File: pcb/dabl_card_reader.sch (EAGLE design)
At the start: 11 parts

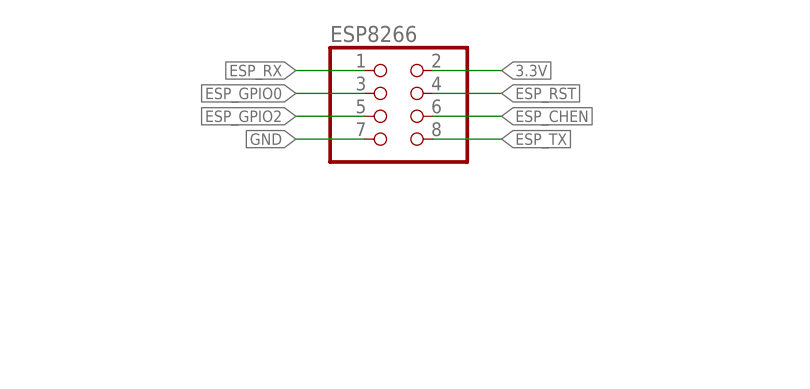
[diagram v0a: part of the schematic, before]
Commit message: fix pcb traces
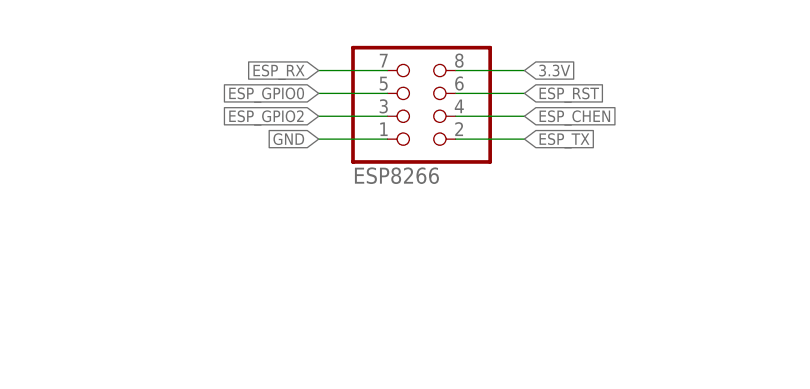
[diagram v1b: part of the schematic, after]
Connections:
- net 3.3V: now also ESP8266.8; no longer ESP8266.2
- net ESP_CHEN: now also ESP8266.4; no longer ESP8266.6
- net ESP_GPIO0: now also ESP8266.5; no longer ESP8266.3
- net ESP_GPIO2: now also ESP8266.3; no longer ESP8266.5
- net ESP_RST: now also ESP8266.6; no longer ESP8266.4
- net ESP_RX: now also ESP8266.7; no longer ESP8266.1
- net ESP_TX: now also ESP8266.2; no longer ESP8266.8
- net GND: now also ESP8266.1; no longer ESP8266.7
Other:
- moved on the sheet: ESP8266
